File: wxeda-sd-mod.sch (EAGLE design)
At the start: 26 parts, among them T1 2N3904, U1 SD_CARD, X1 TV OUT, X2 TAPE IN / OUT

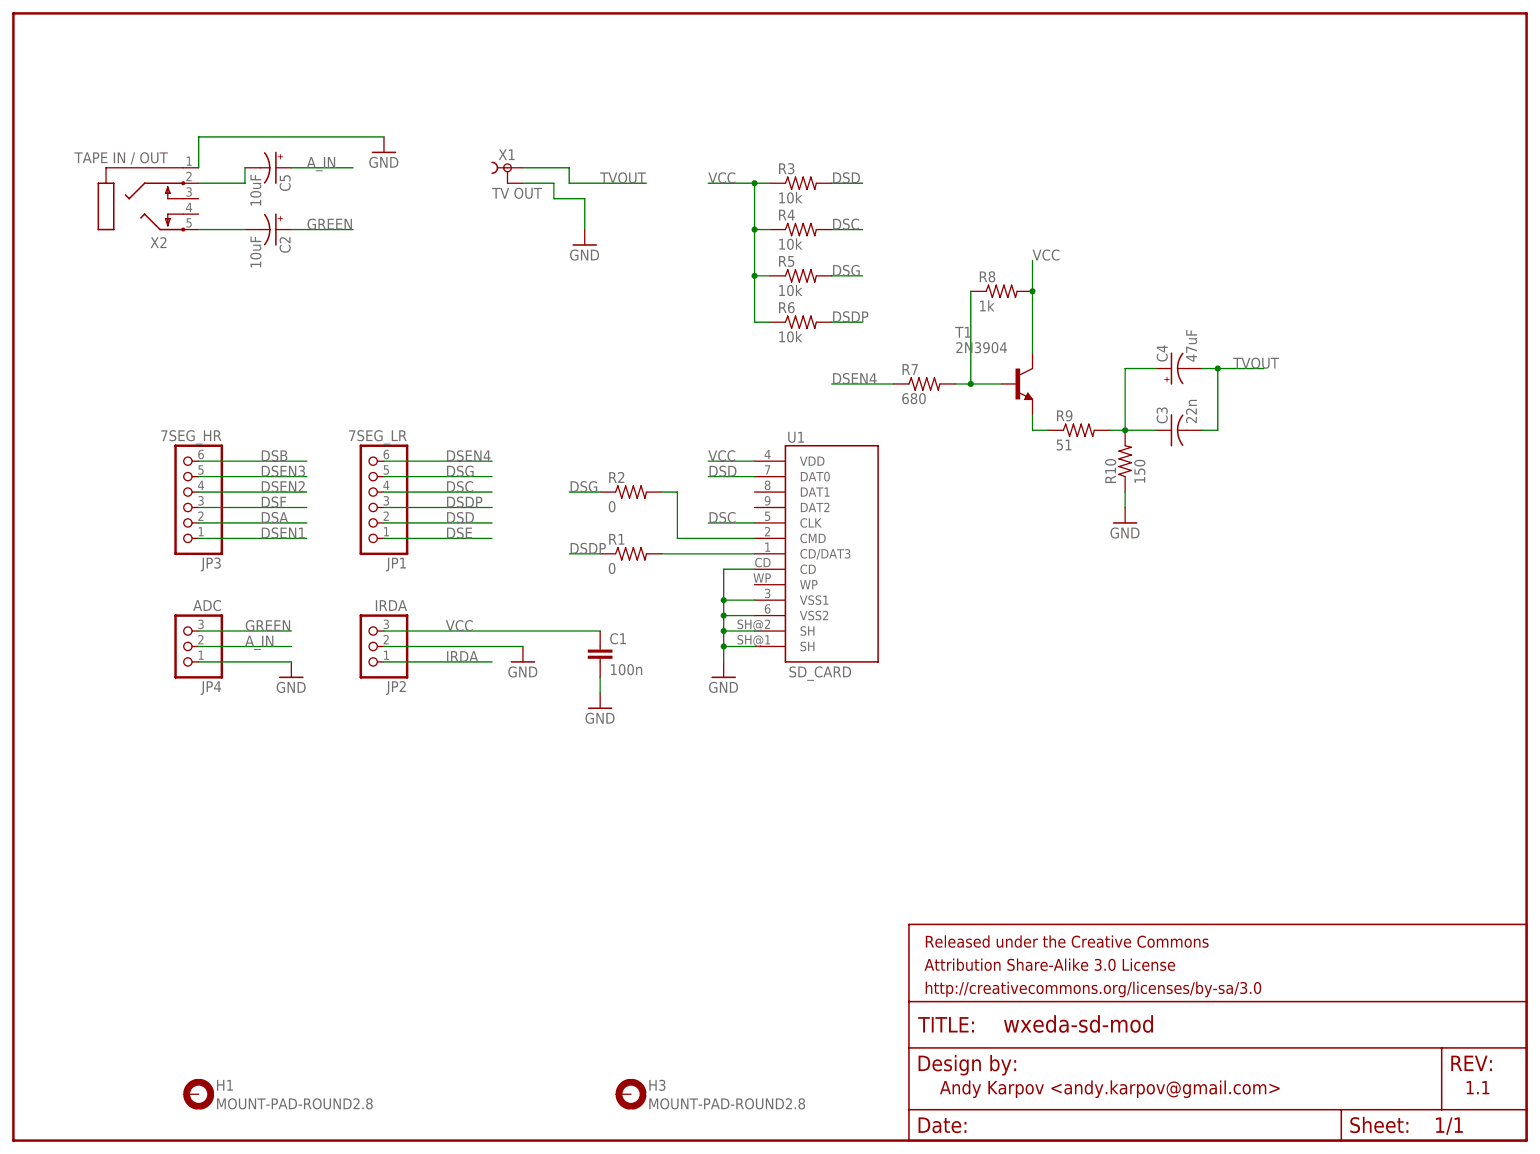
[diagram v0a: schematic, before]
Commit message: minor changes
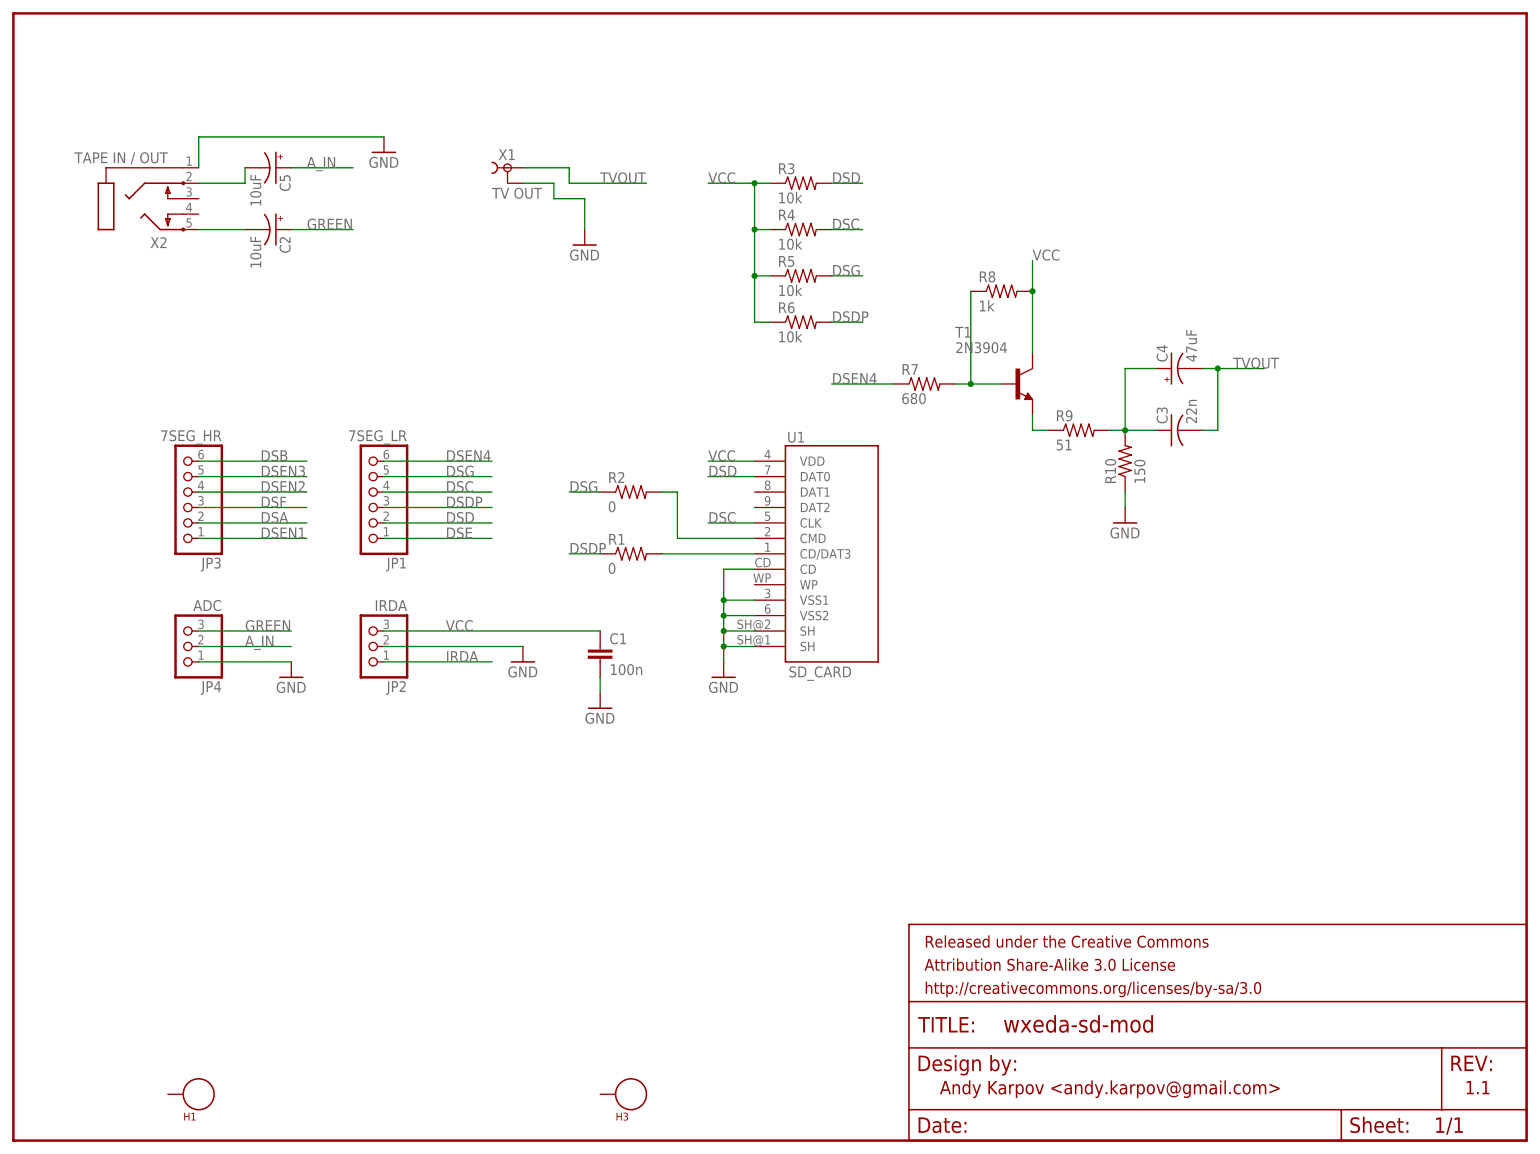
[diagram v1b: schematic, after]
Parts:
- H1, H3: value MOUNT-PAD-ROUND2.8 -> SEW_HOLE; device holes:MOUNT-PAD-ROUND2.8 -> LilyPad-Wearables:SEW_HOLE
- R10, R7, R8, R9: device adafruit:R-US_0204/7 -> SparkFun-Passives:RESISTORAXIAL-0.3
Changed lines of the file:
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@@
 <part name="GND3" library="SparkFun-Aesthetics" deviceset="GND" device=""/>
 <part name="FRAME1" library="SparkFun-Aesthetics" deviceset="FRAME-LETTER" device=""/>
-<part name="H1" library="holes" deviceset="MOUNT-PAD-ROUND" device="2.8"/>
-<part name="H3" library="holes" deviceset="MOUNT-PAD-ROUND" device="2.8"/>
+<part name="H1" library="LilyPad-Wearables" deviceset="SEW_HOLE" device=""/>
+<part name="H3" library="LilyPad-Wearables" deviceset="SEW_HOLE" device=""/>
 <part name="R1" library="SparkFun-Passives" deviceset="RESISTOR" device="AXIAL-0.3" value="0"/>
 <part name="R2" library="SparkFun-Passives" deviceset="RESISTOR" device="AXIAL-0.3" value="0"/>
@@
 <part name="GND7" library="SparkFun-Aesthetics" deviceset="GND" device=""/>
 <part name="T1" library="transistor" deviceset="2N3904" device=""/>
-<part name="R7" library="adafruit" deviceset="R-US_" device="0204/7" value="680"/>
-<part name="R8" library="adafruit" deviceset="R-US_" device="0204/7" value="1k"/>
-<part name="R9" library="adafruit" deviceset="R-US_" device="0204/7" value="51"/>
-<part name="R10" library="adafruit" deviceset="R-US_" device="0204/7" value="150"/>
+<part name="R7" library="SparkFun-Passives" deviceset="RESISTOR" device="AXIAL-0.3" value="680"/>
+<part name="R8" library="SparkFun-Passives" deviceset="RESISTOR" device="AXIAL-0.3" value="1k"/>
+<part name="R9" library="SparkFun-Passives" deviceset="RESISTOR" device="AXIAL-0.3" value="51"/>
+<part name="R10" library="SparkFun-Passives" deviceset="RESISTOR" device="AXIAL-0.3" value="150"/>
 <part name="C3" library="adafruit" deviceset="C-US" device="050-025X075" value="22n"/>
 <part name="C4" library="adafruit" deviceset="CPOL-US" device="E5-8.5" value="47uF"/>
